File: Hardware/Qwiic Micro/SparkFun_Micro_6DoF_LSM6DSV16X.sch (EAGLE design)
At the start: 29 parts, among them J1 Qwiic Right Angle, U2 LSM6DSV16X

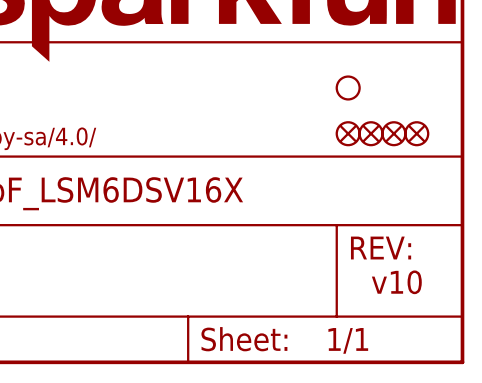
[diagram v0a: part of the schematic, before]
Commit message: Adds proto gerbers
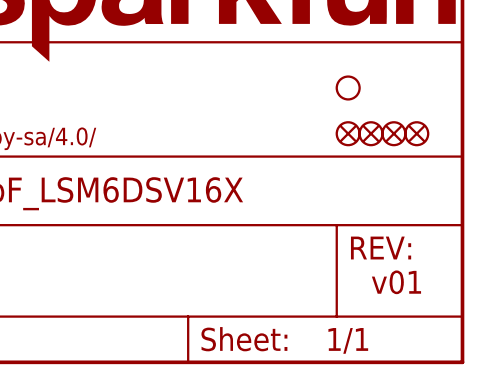
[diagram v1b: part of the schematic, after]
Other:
- note added: "v01"
- note removed: "v10"
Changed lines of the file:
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@@
 <text x="65.786" y="172.974" size="1.27" layer="97" font="vector">VDD Range: 1.71V - 3.6V
 VDDIO Range: 1.62V - 3.6V</text>
-<text x="238.76" y="7.62" size="2.54" layer="94" font="vector">v10</text>
+<text x="238.76" y="7.62" size="2.54" layer="94" font="vector">v01</text>
 <text x="210.82" y="180.34" size="2.54" layer="94" font="vector" align="center">Jumpers</text>
 <text x="213.36" y="132.08" size="1.778" layer="97" font="vector">Cut trace to
